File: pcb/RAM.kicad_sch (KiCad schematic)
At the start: 33 parts, among them U4 MT41K64M16TW-x

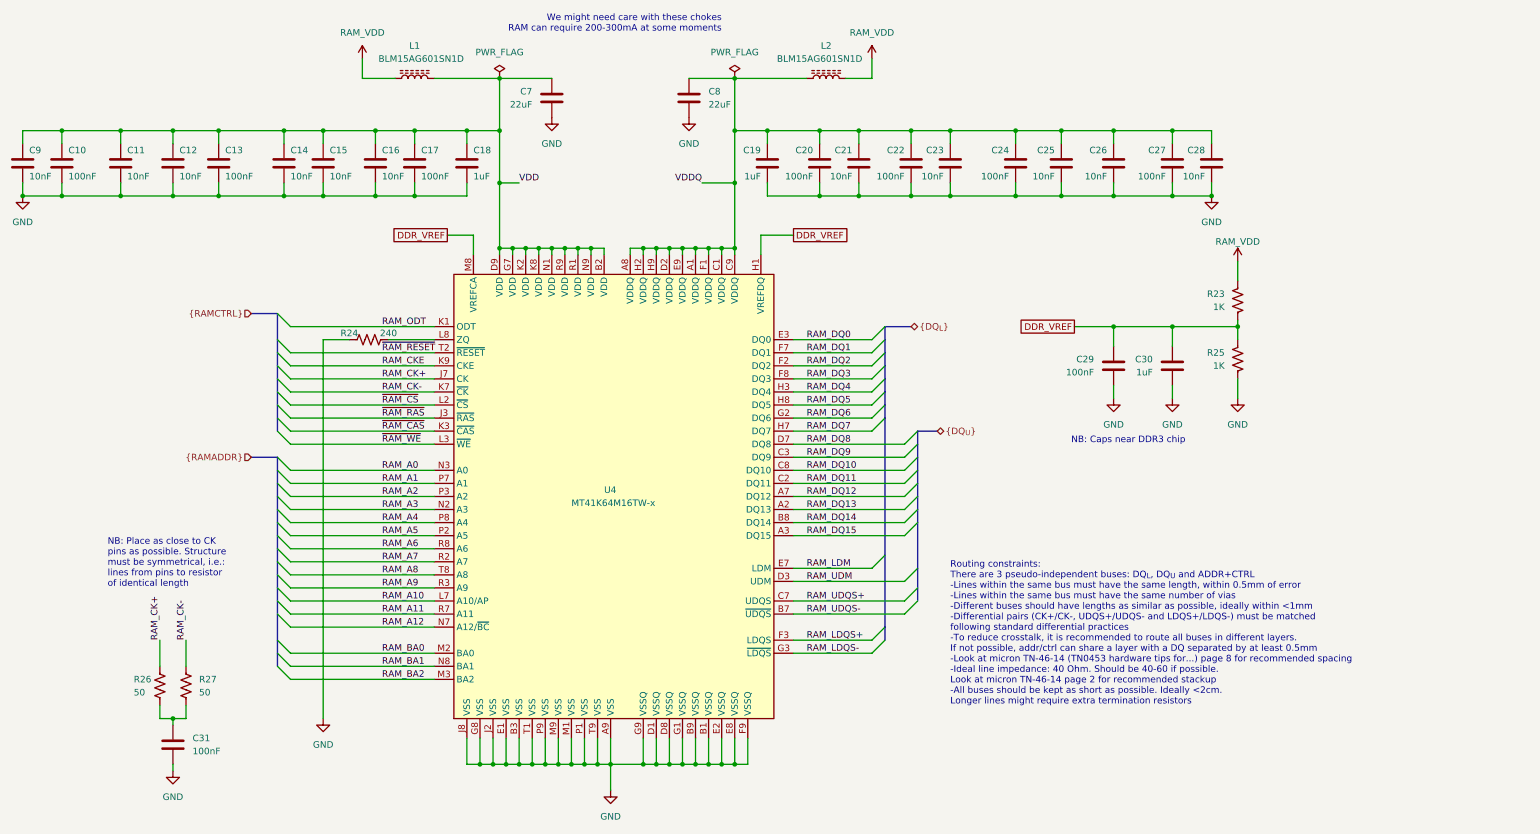
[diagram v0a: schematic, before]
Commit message: Rev. A before fab comments
- Added gerbers, mount positions, etc.
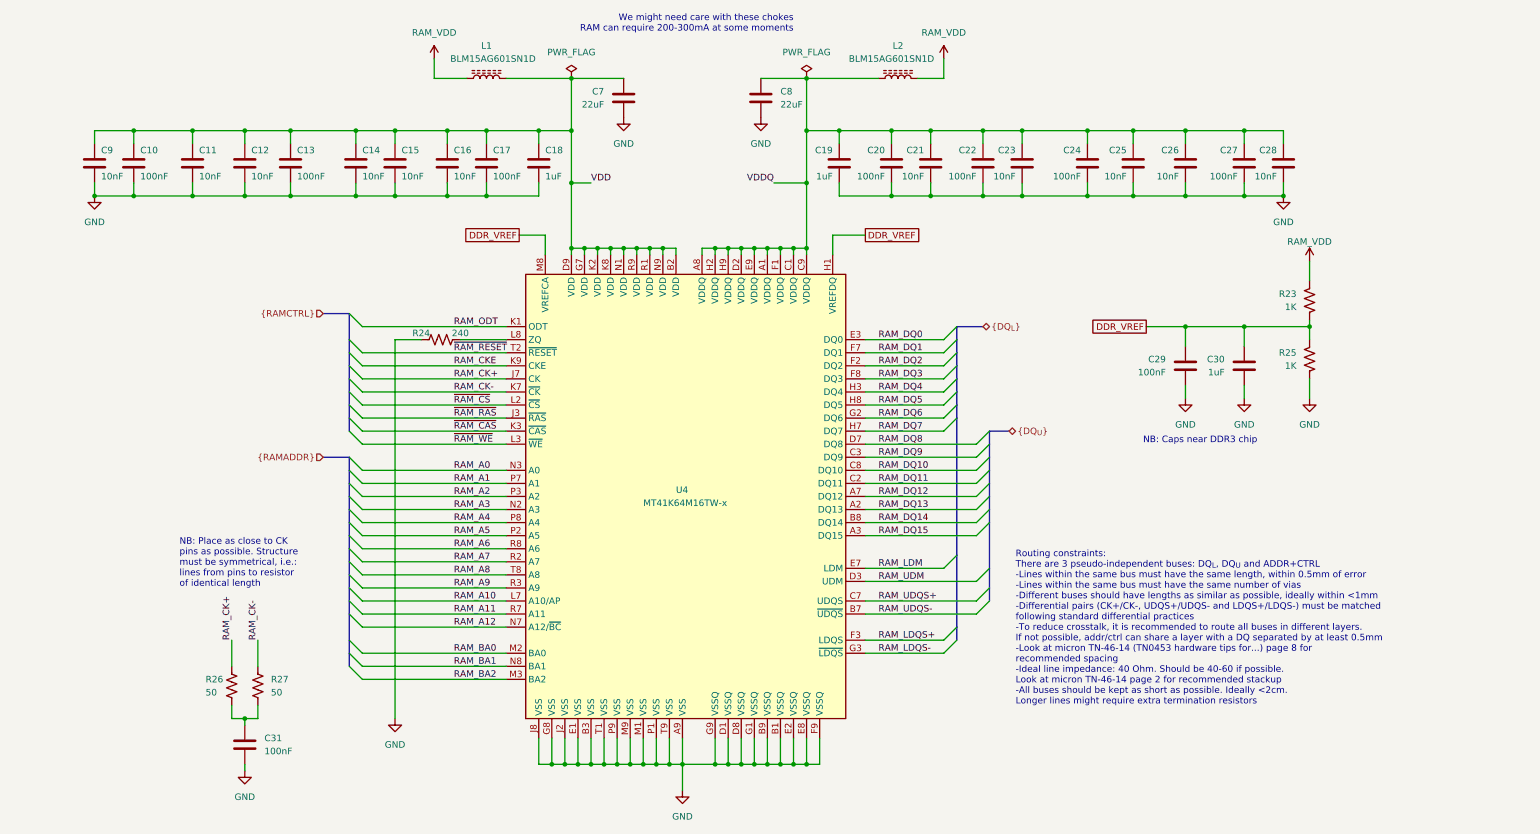
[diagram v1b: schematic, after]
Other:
- moved on the sheet: C10, C11, C12, C13, C14, C15, C16, C17, C18, C19, C20, C21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
